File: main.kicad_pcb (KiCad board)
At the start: 2 copper layers, 4 parts, among them M1 XBEE, U1 BME280, U2 NCS36000

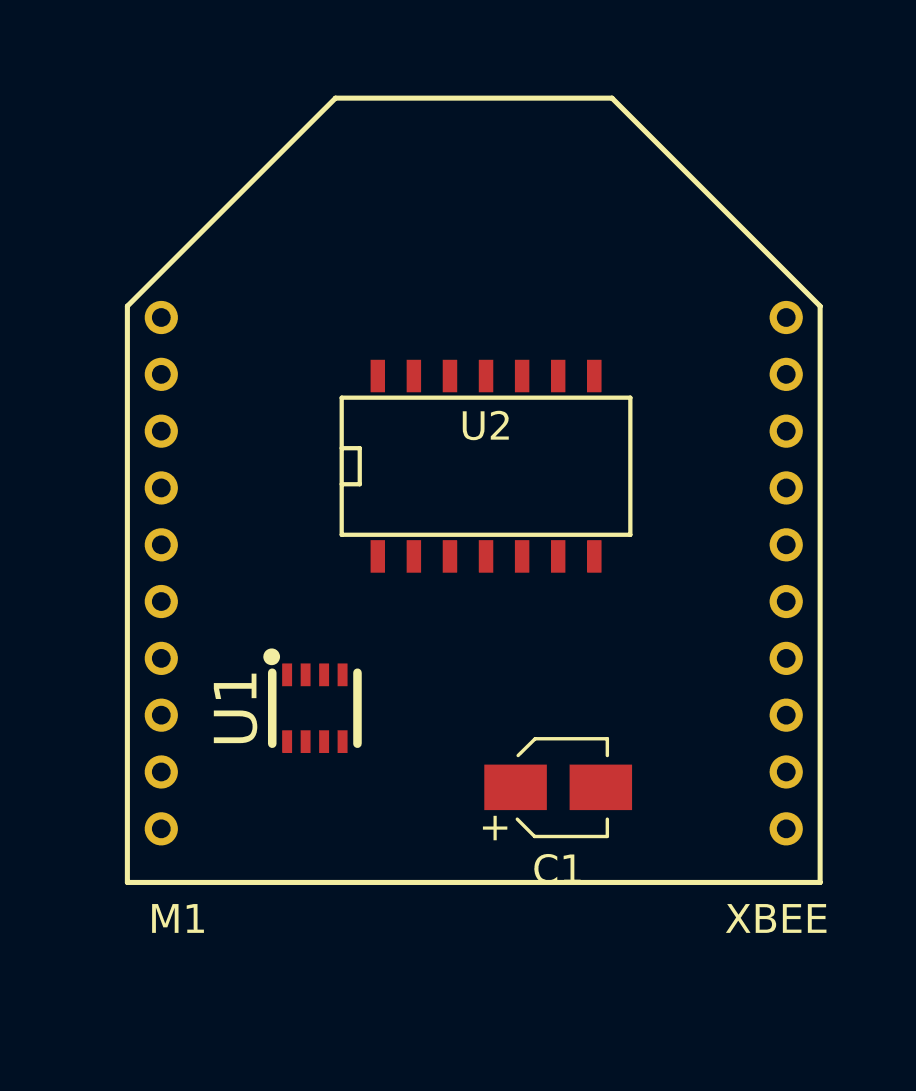
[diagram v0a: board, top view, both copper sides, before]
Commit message: test
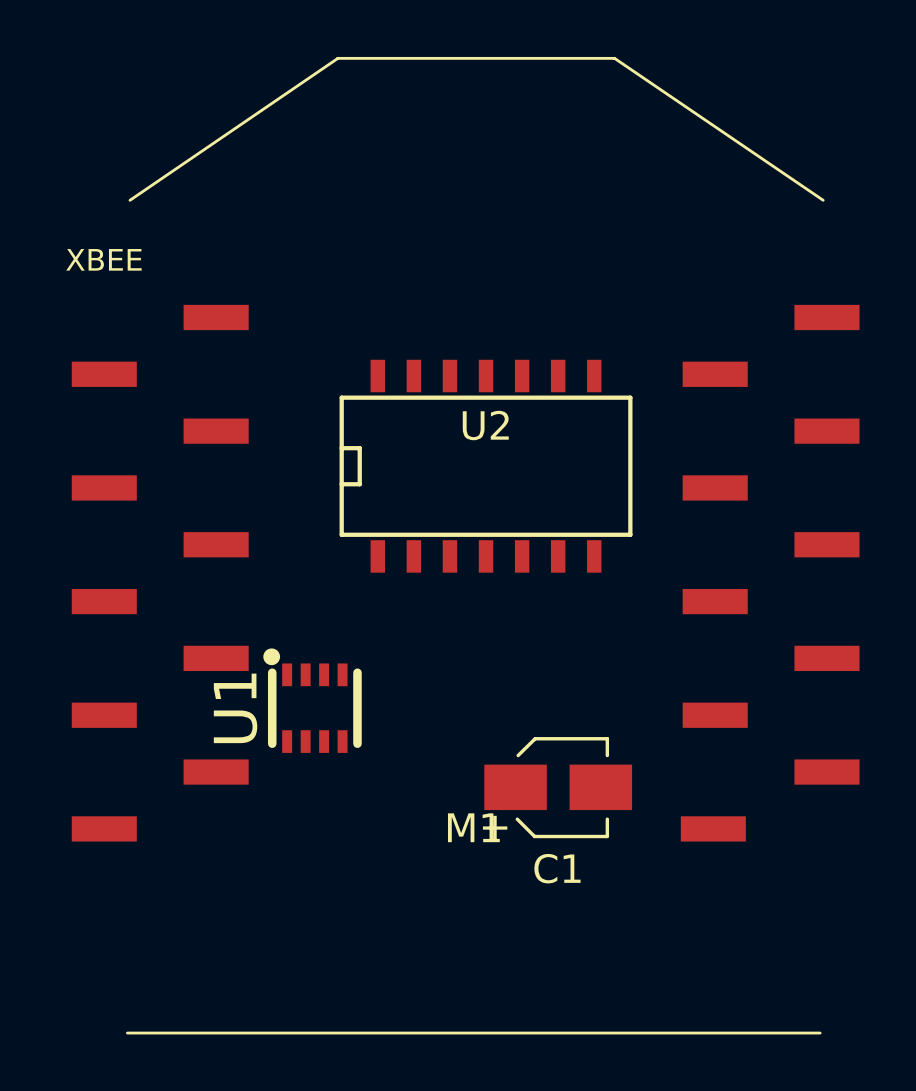
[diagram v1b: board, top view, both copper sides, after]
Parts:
- M1: footprint BME280:XBEE -> XBEE:XBEE-SMD
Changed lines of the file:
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@@
     (links 5)
     (no_connects 5)
-    (area 176.317299 87.211559 201.577248 117.47688)
+    (area 174.165194 85.846309 202.57704 120.658231)
     (thickness 1.6)
     (drawings 0)
@@
     )
   )
-  (module BME280:XBEE (layer F.Cu)
+  (module XBEE:XBEE-SMD (layer F.Cu)
     (at 188.7982 104.22128)
-    (attr virtual)
-    (fp_text reference M1 (at -10.414 12.192) (layer F.SilkS)
+    (attr smd)
+    (fp_text reference M1 (at 0 8.99922) (layer F.SilkS)
       (effects (font (size 1.016 1.016) (thickness 0.1016)))
     )
-    (fp_text value XBEE (at 10.668 12.192) (layer F.SilkS)
-      (effects (font (size 1.016 1.016) (thickness 0.1016)))
-    )
-    (fp_line (start -12.192 10.88644) (end 12.192 10.88644) (layer F.SilkS) (width 0.1778))
-    (fp_line (start 12.192 10.88644) (end 12.192 -9.398) (layer F.SilkS) (width 0.1778))
-    (fp_line (start 12.192 -9.398) (end 4.86664 -16.72082) (layer F.SilkS) (width 0.1778))
-    (fp_line (start 4.86664 -16.72082) (end -4.86664 -16.72082) (layer F.SilkS) (width 0.1778))
-    (fp_line (start -4.86664 -16.72082) (end -12.192 -9.398) (layer F.SilkS) (width 0.1778))
-    (fp_line (start -12.192 -9.398) (end -12.192 10.88644) (layer F.SilkS) (width 0.1778))
-    (fp_line (start -12.192 10.88644) (end 12.192 10.88644) (layer F.SilkS) (width 0.127))
-    (fp_line (start 12.192 10.88644) (end 12.192 -9.398) (layer F.SilkS) (width 0.127))
-    (fp_line (start 12.192 -9.398) (end 4.86664 -16.72082) (layer F.SilkS) (width 0.127))
-    (fp_line (start 4.86664 -16.72082) (end -4.86664 -16.72082) (layer F.SilkS) (width 0.127))
-    (fp_line (start -4.86664 -16.72082) (end -12.192 -9.398) (layer F.SilkS) (width 0.127))
-    (fp_line (start -12.192 -9.398) (end -12.192 10.88644) (layer F.SilkS) (width 0.127))
-    (pad 1 thru_hole circle (at -10.9982 -8.99922) (size 1.1684 1.1684) (drill 0.6604) (layers *.Cu *.Mask F.Paste F.SilkS)
+    (fp_text value XBEE (at -12.99972 -11.00074) (layer F.SilkS)
+      (effects (font (size 0.762 0.762) (thickness 0.1016)))
+    )
+    (fp_line (start 12.30122 -13.12418) (end 4.95046 -18.12544) (layer F.SilkS) (width 0.09906))
+    (fp_line (start -12.10056 -13.12418) (end -4.7752 -18.12544) (layer F.SilkS) (width 0.09906))
+    (fp_line (start -12.192 16.18742) (end 12.192 16.18742) (layer F.SilkS) (width 0.09906))
+    (fp_line (start 4.94284 -18.12036) (end -4.79044 -18.12036) (layer F.SilkS) (width 0.09906))
+    (pad 2 smd rect (at -13.0048 -7.00024 270) (size 0.889 2.29108) (layers F.Cu F.Paste F.Mask)
+      (net 22 "Net-(M1-Pad2)"))
+    (pad 4 smd rect (at -13.0048 -2.99974 270) (size 0.889 2.29108) (layers F.Cu F.Paste F.Mask)
+      (net 24 "Net-(M1-Pad4)"))
+    (pad 6 smd rect (at -13.0048 1.00076 270) (size 0.889 2.29108) (layers F.Cu F.Paste F.Mask)
+      (net 26 "Net-(M1-Pad6)"))
+    (pad 8 smd rect (at -13.0048 5.00126 270) (size 0.889 2.29108) (layers F.Cu F.Paste F.Mask)
+      (net 28 "Net-(M1-Pad8)"))
+    (pad 10 smd rect (at -13.0048 9.00176 270) (size 0.889 2.29108) (layers F.Cu F.Paste F.Mask)
+      (net 1 GND))
+    (pad 9 smd rect (at -9.0678 7.00024 270) (size 0.889 2.29108) (layers F.Cu F.Paste F.Mask)
+      (net 29 "Net-(M1-Pad9)"))
+    (pad 7 smd rect (at -9.0678 2.99974 270) (size 0.889 2.29108) (layers F.Cu F.Paste F.Mask)
+      (net 27 "Net-(M1-Pad7)"))
+    (pad 5 smd rect (at -9.0678 -1.00076 270) (size 0.889 2.29108) (layers F.Cu F.Paste F.Mask)
+      (net 25 "Net-(M1-Pad5)"))
+    (pad 3 smd rect (at -9.0678 -4.99872 270) (size 0.889 2.29108) (layers F.Cu F.Paste F.Mask)
+      (net 23 "Net-(M1-Pad3)"))
+    (pad 1 smd rect (at -9.0678 -8.99922 270) (size 0.889 2.29108) (layers F.Cu F.Paste F.Mask)
       (net 6 +3V3))
-    (pad 2 thru_hole circle (at -10.9982 -6.9977) (size 1.1684 1.1684) (drill 0.6604) (layers *.Cu *.Mask F.Paste F.SilkS)
-      (net 22 "Net-(M1-Pad2)"))
-    (pad 3 thru_hole circle (at -10.9982 -4.99872) (size 1.1684 1.1684) (drill 0.6604) (layers *.Cu *.Mask F.Paste F.SilkS)
-      (net 23 "Net-(M1-Pad3)"))
-    (pad 4 thru_hole circle (at -10.9982 -2.99974) (size 1.1684 1.1684) (drill 0.6604) (layers *.Cu *.Mask F.Paste F.SilkS)
-      (net 24 "Net-(M1-Pad4)"))
-    (pad 5 thru_hole circle (at -10.9982 -0.99822) (size 1.1684 1.1684) (drill 0.6604) (layers *.Cu *.Mask F.Paste F.SilkS)
-      (net 25 "Net-(M1-Pad5)"))
-    (pad 6 thru_hole circle (at -10.9982 0.99822) (size 1.1684 1.1684) (drill 0.6604) (layers *.Cu *.Mask F.Paste F.SilkS)
-      (net 26 "Net-(M1-Pad6)"))
-    (pad 7 thru_hole circle (at -10.9982 2.99974) (size 1.1684 1.1684) (drill 0.6604) (layers *.Cu *.Mask F.Paste F.SilkS)
-      (net 27 "Net-(M1-Pad7)"))
-    (pad 8 thru_hole circle (at -10.9982 4.99872) (size 1.1684 1.1684) (drill 0.6604) (layers *.Cu *.Mask F.Paste F.SilkS)
-      (net 28 "Net-(M1-Pad8)"))
-    (pad 9 thru_hole circle (at -10.9982 6.9977) (size 1.1684 1.1684) (drill 0.6604) (layers *.Cu *.Mask F.Paste F.SilkS)
-      (net 29 "Net-(M1-Pad9)"))
-    (pad 10 thru_hole circle (at -10.9982 8.99922) (size 1.1684 1.1684) (drill 0.6604) (layers *.Cu *.Mask F.Paste F.SilkS)
-      (net 1 GND))
-    (pad 11 thru_hole circle (at 10.9982 8.99922) (size 1.1684 1.1684) (drill 0.6604) (layers *.Cu *.Mask F.Paste F.SilkS)
+    (pad 20 smd rect (at 12.4333 -8.99922 270) (size 0.889 2.29108) (layers F.Cu F.Paste F.Mask)
+      (net 39 "Net-(M1-Pad20)"))
+    (pad 19 smd rect (at 8.49884 -7.00024 270) (size 0.889 2.29108) (layers F.Cu F.Paste F.Mask)
+      (net 38 "Net-(M1-Pad19)"))
+    (pad 18 smd rect (at 12.4333 -4.99872 270) (size 0.889 2.29108) (layers F.Cu F.Paste F.Mask)
+      (net 37 "Net-(M1-Pad18)"))
+    (pad 17 smd rect (at 8.49884 -2.99974 270) (size 0.889 2.29108) (layers F.Cu F.Paste F.Mask)
+      (net 36 "Net-(M1-Pad17)"))
+    (pad 16 smd rect (at 12.4333 -1.00076 270) (size 0.889 2.29108) (layers F.Cu F.Paste F.Mask)
+      (net 35 "Net-(M1-Pad16)"))
+    (pad 15 smd rect (at 8.49884 1.00076 270) (size 0.889 2.29108) (layers F.Cu F.Paste F.Mask)
+      (net 34 "Net-(M1-Pad15)"))
+    (pad 14 smd rect (at 12.4333 2.99974 270) (size 0.889 2.29108) (layers F.Cu F.Paste F.Mask)
+      (net 33 "Net-(M1-Pad14)"))
+    (pad 13 smd rect (at 8.49884 5.00126 270) (size 0.889 2.29108) (layers F.Cu F.Paste F.Mask)
+      (net 32 "Net-(M1-Pad13)"))
+    (pad 12 smd rect (at 12.4333 7.00024 270) (size 0.889 2.29108) (layers F.Cu F.Paste F.Mask)
+      (net 31 "Net-(M1-Pad12)"))
+    (pad 11 smd rect (at 8.4328 9.00176 270) (size 0.889 2.29108) (layers F.Cu F.Paste F.Mask)
       (net 30 "Net-(M1-Pad11)"))
-    (pad 12 thru_hole circle (at 10.9982 6.9977) (size 1.1684 1.1684) (drill 0.6604) (layers *.Cu *.Mask F.Paste F.SilkS)
-      (net 31 "Net-(M1-Pad12)"))
-    (pad 13 thru_hole circle (at 10.9982 4.99872) (size 1.1684 1.1684) (drill 0.6604) (layers *.Cu *.Mask F.Paste F.SilkS)
-      (net 32 "Net-(M1-Pad13)"))
-    (pad 14 thru_hole circle (at 10.9982 2.99974) (size 1.1684 1.1684) (drill 0.6604) (layers *.Cu *.Mask F.Paste F.SilkS)
-      (net 33 "Net-(M1-Pad14)"))
-    (pad 15 thru_hole circle (at 10.9982 0.99822) (size 1.1684 1.1684) (drill 0.6604) (layers *.Cu *.Mask F.Paste F.SilkS)
-      (net 34 "Net-(M1-Pad15)"))
-    (pad 16 thru_hole circle (at 10.9982 -0.99822) (size 1.1684 1.1684) (drill 0.6604) (layers *.Cu *.Mask F.Paste F.SilkS)
-      (net 35 "Net-(M1-Pad16)"))
-    (pad 17 thru_hole circle (at 10.9982 -2.99974) (size 1.1684 1.1684) (drill 0.6604) (layers *.Cu *.Mask F.Paste F.SilkS)
-      (net 36 "Net-(M1-Pad17)"))
-    (pad 18 thru_hole circle (at 10.9982 -4.99872) (size 1.1684 1.1684) (drill 0.6604) (layers *.Cu *.Mask F.Paste F.SilkS)
-      (net 37 "Net-(M1-Pad18)"))
-    (pad 19 thru_hole circle (at 10.9982 -6.9977) (size 1.1684 1.1684) (drill 0.6604) (layers *.Cu *.Mask F.Paste F.SilkS)
-      (net 38 "Net-(M1-Pad19)"))
-    (pad 20 thru_hole circle (at 10.9982 -8.99922) (size 1.1684 1.1684) (drill 0.6604) (layers *.Cu *.Mask F.Paste F.SilkS)
-      (net 39 "Net-(M1-Pad20)"))
   )
 )
